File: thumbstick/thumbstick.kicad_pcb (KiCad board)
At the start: 2 copper layers, 30 x 30 mm, 3 parts, among them P1 rkjxv1220001

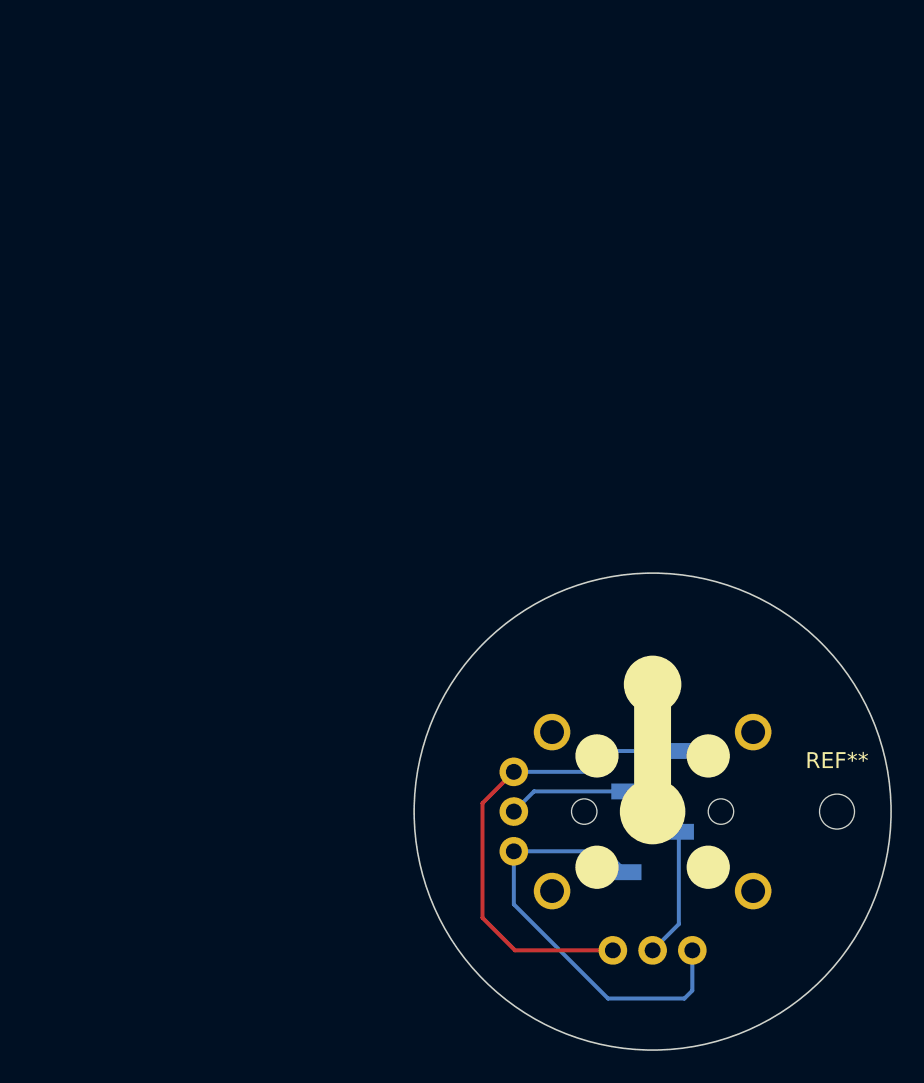
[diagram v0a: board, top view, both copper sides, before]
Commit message: Thubmstick v1
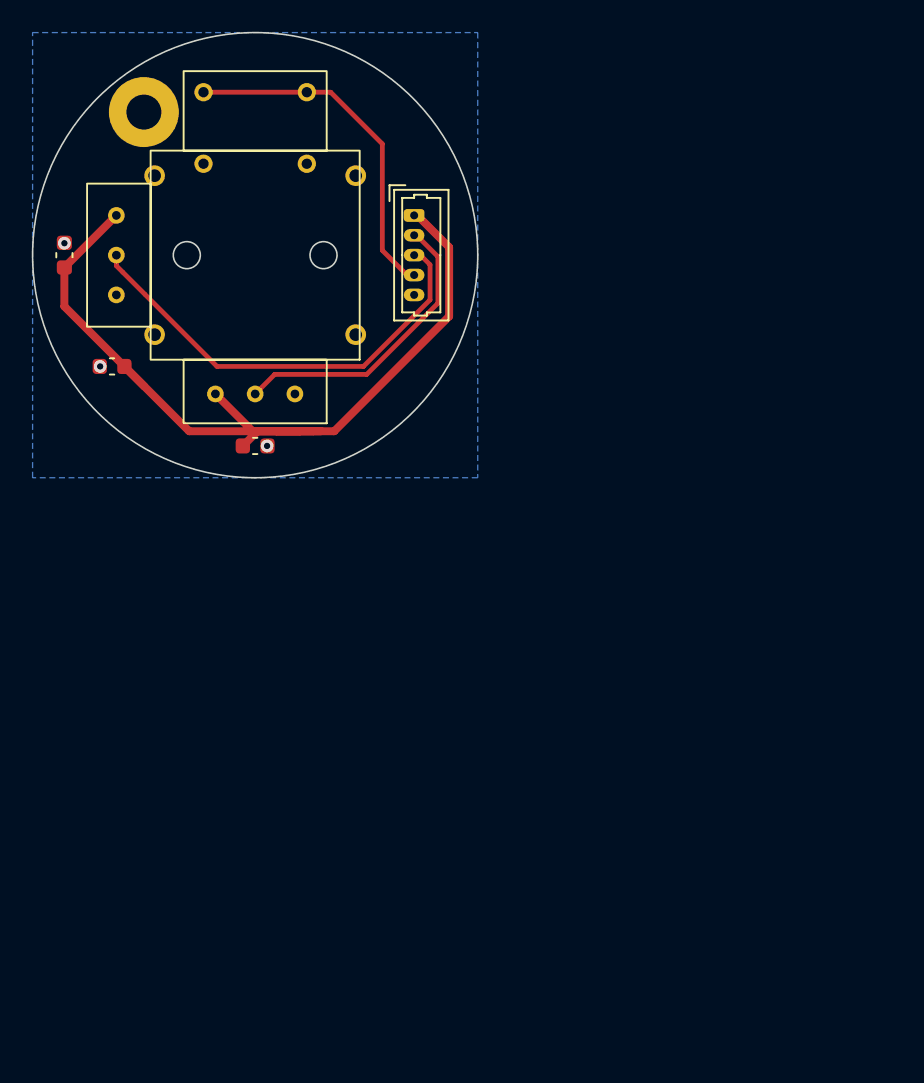
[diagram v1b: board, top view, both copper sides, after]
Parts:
- removed P1: rkjxv1220001, rkjxv1220001:rkjxv1220001
- removed REF**: MountingHole_2.2mm_M2, MountingHole:MountingHole_2.2mm_M2
- removed out1: Conn_01x04_Female, Connector_PinSocket_2.54mm:PinSocket_1x04_P2.54mm_Vertical_SMD_Pin1Left
- added C1: 10uF, Capacitor_SMD:C_0603_1608Metric, F.Cu at (91.0, 72.0)
- added C2: 100nF, Capacitor_SMD:C_0603_1608Metric, F.Cu at (88.0, 65.0)
- added C3: 100nF, Capacitor_SMD:C_0603_1608Metric, F.Cu at (100.0, 77.0)
- added H1: Conn_01x05, Connector_Molex:Molex_PicoBlade_53047-0510_1x05_P1.25mm_Vertical, F.Cu at (110.0, 62.5)
- added MNT1: MountingHole, MountingHole:MountingHole_2.2mm_M2_Pad, F.Cu at (93.0, 56.0)
- added POT1: RKJXV122400R, rkjxv1220001:RKJXV122400R, F.Cu at (100.0, 65.0)
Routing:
- net VCC: track 30.0 -> 60.6 mm
- net Y_OUT: track 0.00 -> 28.2 mm
- net GND: track 27.4 -> 0.00 mm, vias 0 -> 3
- net P_OUT: track 0.00 -> 21.9 mm
- net X_OUT: track 0.00 -> 18.8 mm
- net HORIZ: track 8.14 -> 0.00 mm
- net VERT: track 7.61 -> 0.00 mm
- added copper zone on B.Cu, net GND
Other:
- board size 30 x 30 mm -> 28 x 28 mm
